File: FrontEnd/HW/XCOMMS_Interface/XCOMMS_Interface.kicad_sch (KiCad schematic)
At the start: 18 parts, among them J1 TFC-110-02-F-D-A-P-FR, J2 UART, J3 JTAG, J4 12V, U1 STM32L431KBUx, Y1 TCXO_ECS

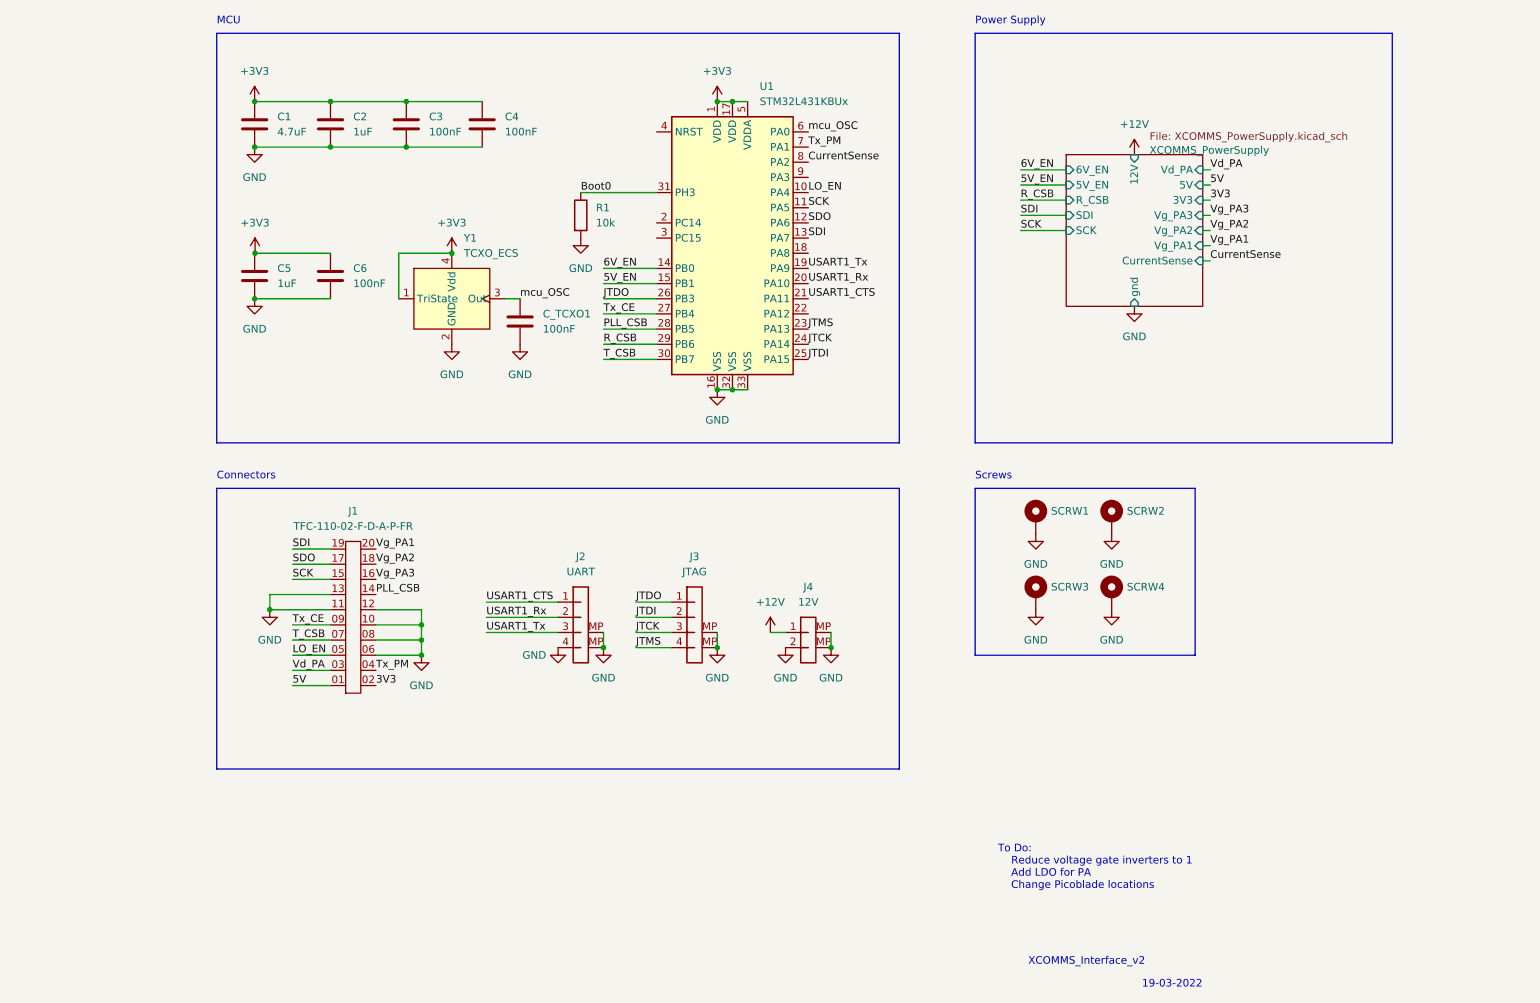
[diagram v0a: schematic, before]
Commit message: XCOMMS Interface rebuild
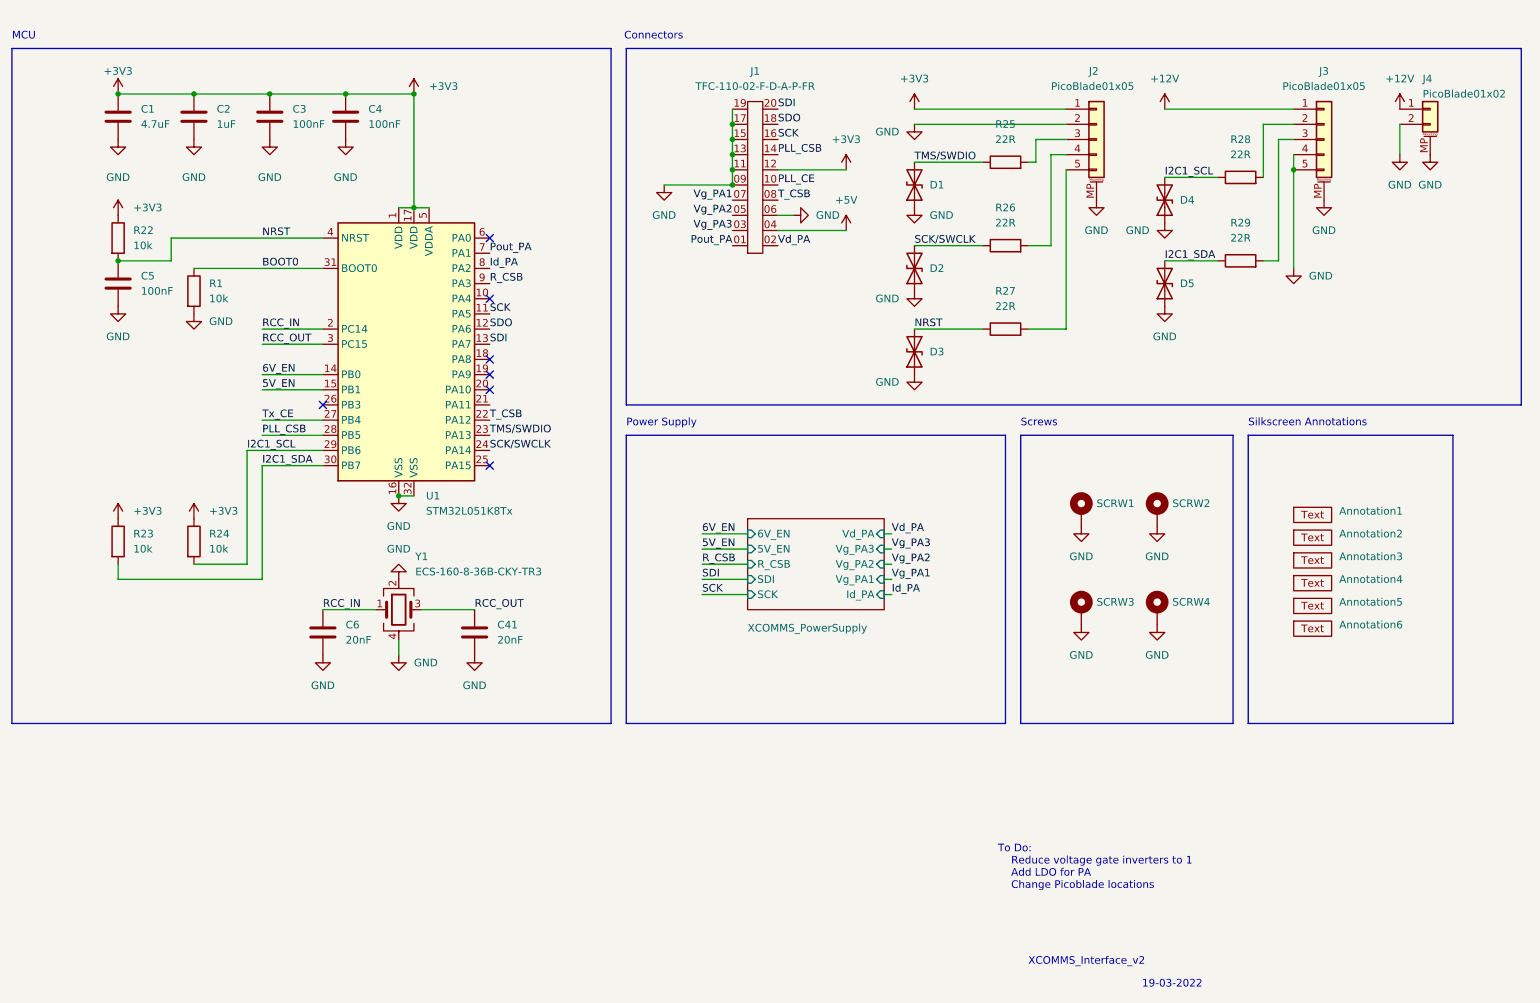
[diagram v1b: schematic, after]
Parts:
- removed C_TCXO1: 100nF, Capacitor_SMD:C_0603_1608Metric, symbol Device:C
- removed J2: UART, Connector_Molex:Molex_PicoBlade_53261-0471_1x04-1MP_P1.25mm_Horizontal, symbol GGS_Connectors:Picoblade_4x1_H
- removed J3: JTAG, Connector_Molex:Molex_PicoBlade_53261-0471_1x04-1MP_P1.25mm_Horizontal, symbol GGS_Connectors:Picoblade_4x1_H
- removed J4: 12V, Connector_Molex:Molex_PicoBlade_53261-0271_1x02-1MP_P1.25mm_Horizontal, symbol GGS_Connectors:Picoblade_2x1_H
- removed U1: STM32L431KBUx, Package_DFN_QFN:QFN-32-1EP_5x5mm_P0.5mm_EP3.45x3.45mm, symbol MCU_ST_STM32L4:STM32L431KBUx
- removed Y1: TCXO_ECS, GGS_Miscellaneous:TCXO_ECS, symbol GGS_Miscellaneous:TCXO_ECS
- added Annotation1: Silkscreen_Annotation, GGS_Symbols:Bike, symbol GGS_Symbols:Silkscreen_Annotation
- added Annotation2: Silkscreen_Annotation, GGS_Symbols:GGS, symbol GGS_Symbols:Silkscreen_Annotation
- added Annotation3: Silkscreen_Annotation, GGS_Symbols:NSL, symbol GGS_Symbols:Silkscreen_Annotation
- added Annotation4: Silkscreen_Annotation, GGS_Symbols:Prj, symbol GGS_Symbols:Silkscreen_Annotation
- added Annotation5: Silkscreen_Annotation, GGS_Symbols:Rev, symbol GGS_Symbols:Silkscreen_Annotation
- added Annotation6: Silkscreen_Annotation, GGS_Symbols:UPC, symbol GGS_Symbols:Silkscreen_Annotation
- added C41: 20nF, Capacitor_SMD:C_0603_1608Metric, symbol Device:C
- added D1, D2, D3, D4, D5: SZESD9X3.3ST5G, Diode_SMD:D_SOD-923, symbol Device:D_TVS
- added J2, J3: PicoBlade01x05, Connector_Molex:Molex_PicoBlade_53261-0571_1x05-1MP_P1.25mm_Horizontal, symbol Connector_Generic_MountingPin:Conn_01x05_MountingPin
- added J4: PicoBlade01x02, Connector_Molex:Molex_PicoBlade_53261-0271_1x02-1MP_P1.25mm_Horizontal, symbol Connector_Generic_MountingPin:Conn_01x02_MountingPin
- added R22, R23, R24: 10k, Resistor_SMD:R_0603_1608Metric, symbol Device:R
- added R25, R26, R27, R28, R29: 22R, Resistor_SMD:R_0603_1608Metric, symbol Device:R
- added U1: STM32L051K8Tx, Package_QFP:LQFP-32_7x7mm_P0.8mm, symbol MCU_ST_STM32L0:STM32L051K8Tx
- added Y1: ECS-160-8-36B-CKY-TR3, Oscillator:Oscillator_SMD_ECS_2520MV-xxx-xx-4Pin_2.5x2.0mm, symbol Device:Crystal_GND24
- C1: footprint Capacitor_SMD:C_0805_2012Metric -> Capacitor_SMD:C_0603_1608Metric
- C5: value 1uF -> 100nF
- C6: value 100nF -> 20nF
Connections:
- net 3V3 is gone; now on net Vd_PA: J1.02
- net LO_EN is gone; now on net Vg_PA2: J1.05
- net +12V: now also J3.1 (Pin_1), J4.1 (Pin_1)
- net +3V3: now also J1.12, J2.1 (Pin_1), R22.1, R23.1, R24.1, U1.1 (VDD), U1.17 (VDD), U1.5 (VDDA); no longer C5.1, C6.1
- net 5V_EN: now also U1.15 (PB1)
- net 6V_EN: now also U1.14 (PB0)
- net GND: now also J1.09, J1.15, J1.17, J1.19, C41.2, D1.1 (A1), D2.1 (A1), D3.1 (A1), D4.1 (A1), D5.1 (A1), J2.2 (Pin_2), J2.MP (MountPin), J3.4 (Pin_4), J3.5 (Pin_5), J3.MP (MountPin), J4.2 (Pin_2), J4.MP (MountPin), U1.16 (VSS), U1.32 (VSS), Y1.2, Y1.4; no longer J1.08, J1.10, J1.12
- net PLL_CSB: now also U1.28 (PB5)
- net R_CSB: now also U1.9 (PA3)
- net SCK: now also J1.16, U1.11 (PA5); no longer J1.15
- net SDI: now also J1.20, U1.13 (PA7); no longer J1.19
- net SDO: now also J1.18, U1.12 (PA6); no longer J1.17
- net T_CSB: now also J1.08, U1.22 (PA12); no longer J1.07
- net Tx_CE: now also U1.27 (PB4); no longer J1.09
- net Vd_PA: no longer J1.03
- net Vg_PA1: now also J1.07; no longer J1.20
- net Vg_PA2: no longer J1.18
- net Vg_PA3: now also J1.03; no longer J1.16
- net 5V renamed Pout_PA
- net Pout_PA: now also U1.7 (PA1)
- net Boot0 renamed BOOT0
- net BOOT0: now also U1.31 (BOOT0)
- net Tx_PM renamed +5V
- new net: J2.3 (Pin_3), R25.2
- new net: J2.5 (Pin_5), R27.2
- new net: J3.2 (Pin_2), R28.2
- new net: J2.4 (Pin_4), R26.2
- new net: J3.3 (Pin_3), R29.2
- new net I2C1_SCL: D4.2 (A2), R24.2, R28.1, U1.29 (PB6)
- new net I2C1_SDA: D5.2 (A2), R23.2, R29.1, U1.30 (PB7)
- new net Id_PA: U1.8 (PA2)
- new net NRST: C5.1, D3.2 (A2), R22.2, R27.1, U1.4 (NRST)
- new net PLL_CE: J1.10
- new net RCC_IN: C6.1, U1.2 (PC14), Y1.1
- new net RCC_OUT: C41.1, U1.3 (PC15), Y1.3
- new net SCK/SWCLK: D2.2 (A2), R26.1, U1.24 (PA14)
- new net TMS/SWDIO: D1.2 (A2), R25.1, U1.23 (PA13)
- no-connect marks 0 -> 7
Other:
- sheet XCOMMS_PowerSupply ports: added Id_PA; removed 12V, 3V3, 5V, CurrentSense, gnd
- note added: "Silkscreen Annotations"
- moved on the sheet: C1, C2, C3, C4, J1, SCRW1, SCRW2, SCRW3, SCRW4
